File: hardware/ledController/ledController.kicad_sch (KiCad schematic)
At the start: 8 parts, among them IC1 PIC16F1769-I_ML, J1 Conn_01x06

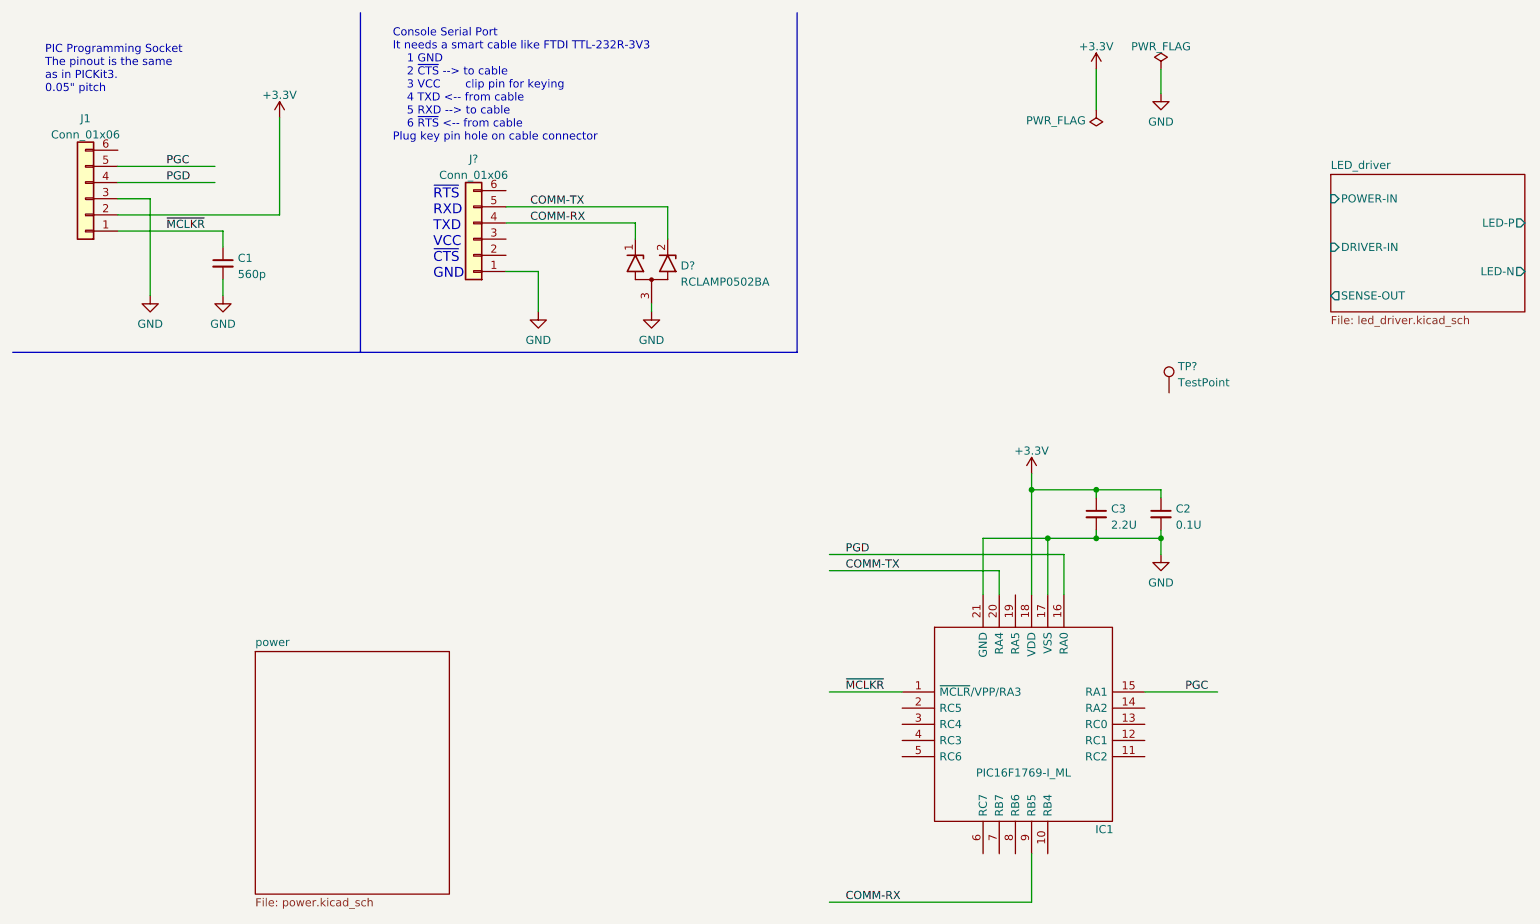
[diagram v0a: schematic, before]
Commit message: Putting everything together
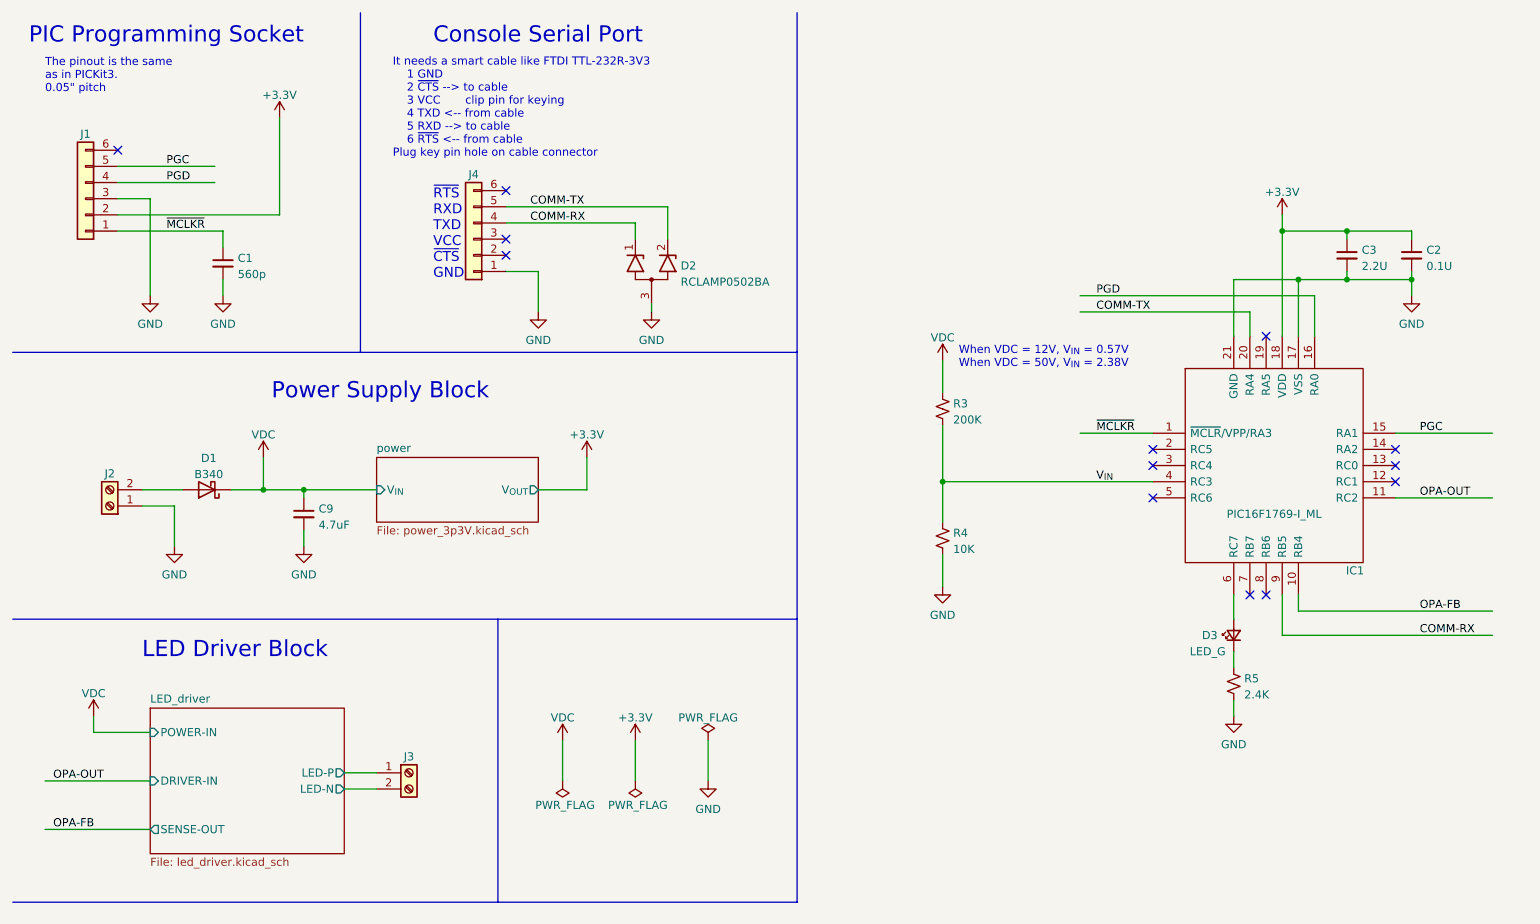
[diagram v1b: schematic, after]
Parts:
- removed TP?: TestPoint, symbol Connector:TestPoint
- added C9: 4.7uF, Capacitor_SMD:C_0402_1005Metric_Pad0.74x0.62mm_HandSolder, symbol Device:C_Small
- added D1: B340, Diode_SMD:D_SMC, symbol Diode:B340
- added D3: LED_G, symbol Device:LED_Small
- added J2, J3: Screw_Terminal_01x02, symbol Connector:Screw_Terminal_01x02
- added R3: 200K, Resistor_SMD:R_0603_1608Metric_Pad0.98x0.95mm_HandSolder, symbol Device:R_Small_US
- added R4: 10K, Resistor_SMD:R_0603_1608Metric_Pad0.98x0.95mm_HandSolder, symbol Device:R_Small_US
- added R5: 2.4K, Resistor_SMD:R_0603_1608Metric_Pad0.98x0.95mm_HandSolder, symbol Device:R_Small_US
- gave numbers to parts that had none: 2
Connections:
- net GND: now also C9.2, J2.1 (Pin_1), R4.2, R5.2
- net LED_driver/LED-N: now also J3.2 (Pin_2)
- net LED_driver/LED-P: now also J3.1 (Pin_1)
- net OPA-FB: now reaches IC1.10 (RB4)
- net OPA-OUT: now reaches IC1.11 (RC2)
- net V_{IN}: now reaches IC1.4 (RC3)
- net V_{IN}: now also R3.2, R4.1
- net at IC1.6 (RC7): now also D3.2 (A)
- new net: D1.2 (A), J2.2 (Pin_2)
- new net: D3.1 (K), R5.1
- new net VDC: C9.1, D1.1 (K), R3.1
- no-connect marks 0 -> 13
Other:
- sheet power: file power.kicad_sch -> power_3p3V.kicad_sch
- sheet power ports: added V_{IN}, V_{OUT}; removed none
- note added: "Console Serial Port"
- note added: "It needs a smart cable like FTDI TTL-232R-3V3 1 GND 2 ~{CTS} --> to cable 3 VCC clip pin for keying 4 TXD <-- from cable 5 RXD --> to cable 6 ~{RTS} <-- from cable Plug key pin hole on cable connector"
- note added: "LED Driver Block"
- note added: "PIC Programming Socket"
- note added: "Power Supply Block"
- note added: "The pinout is the same as in PICKit3. 0.05" pitch"
- note added: "When VDC = 12V, V_{IN} = 0.57V When VDC = 50V, V_{IN} = 2.38V"
- note removed: "Console Serial Port It needs a smart cable like FTDI TTL-232R-3V3 1 GND 2 ~{CTS} --> to cable 3 VCC clip pin for keying 4 TXD <-- from cable 5 RXD --> to cable 6 ~{RTS} <-- from cable Plug key pin hole on cable connector"
- note removed: "PIC Programming Socket The pinout is the same as in PICKit3. 0.05" pitch"
- title: (none) -> Lantern
- moved on the sheet: C2, C3, IC1
